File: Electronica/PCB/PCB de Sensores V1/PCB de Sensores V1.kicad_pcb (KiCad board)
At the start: 2 copper layers, 64.3 x 32.9 mm, 11 parts

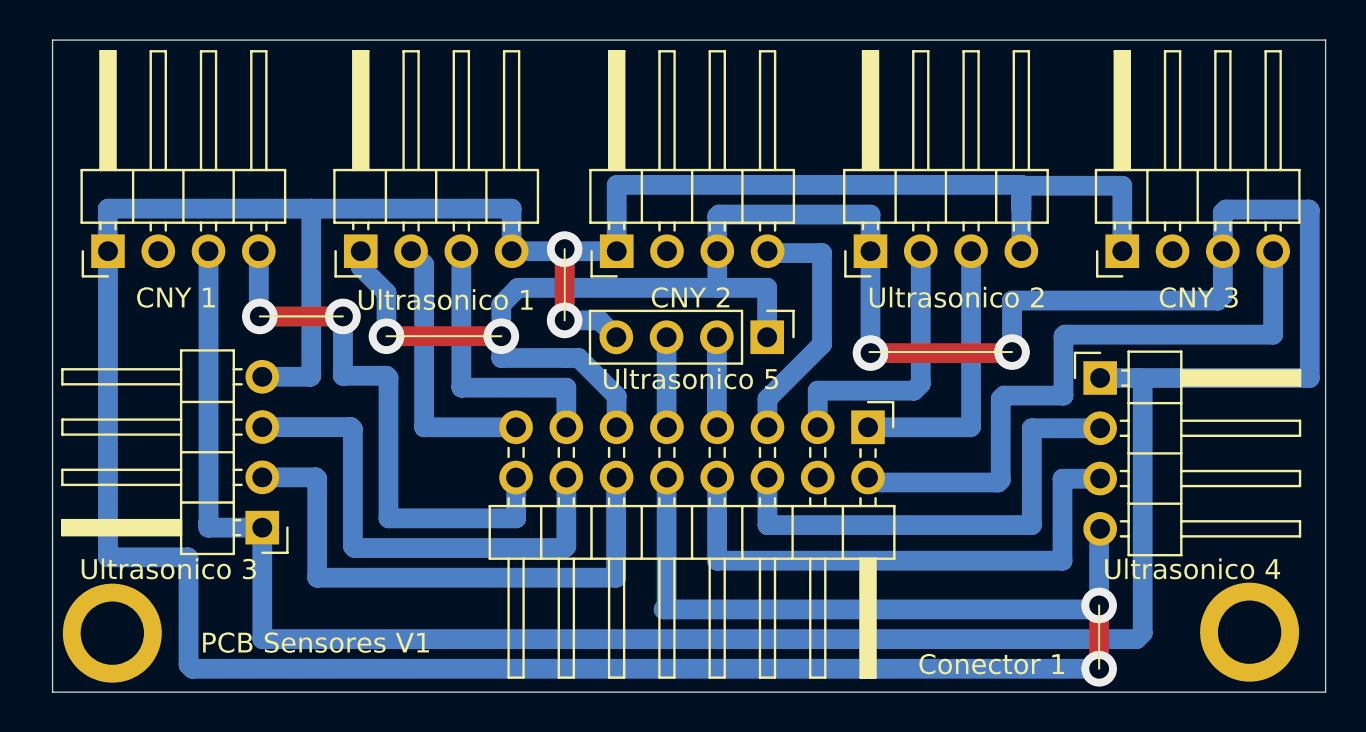
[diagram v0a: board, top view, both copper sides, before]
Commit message: ?
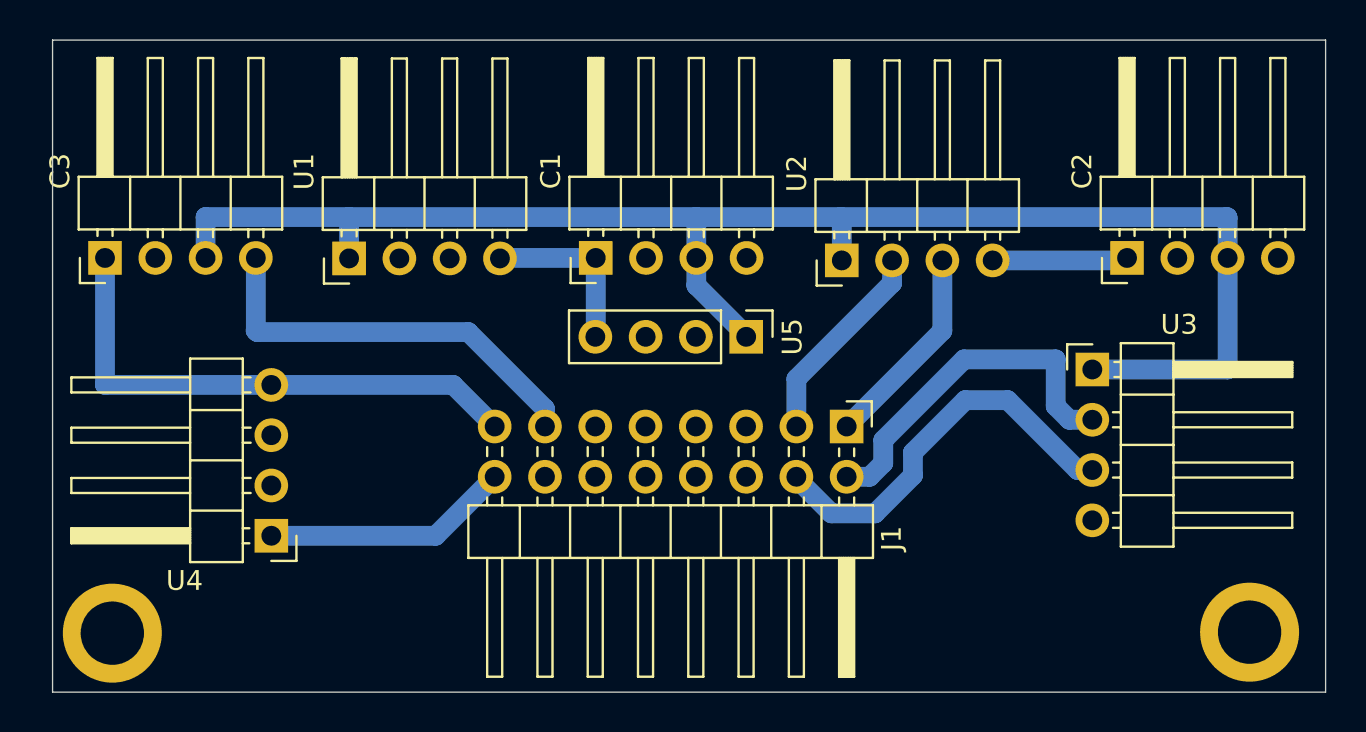
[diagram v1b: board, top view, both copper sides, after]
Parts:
- removed CNY 1: CNY1, Connector_PinHeader_2.54mm:PinHeader_1x04_P2.54mm_Horizontal
- removed CNY 2: CNY2, Connector_PinHeader_2.54mm:PinHeader_1x04_P2.54mm_Horizontal
- removed CNY 3: CNY3, Connector_PinHeader_2.54mm:PinHeader_1x04_P2.54mm_Horizontal
- removed Conector 1: Conn_02x08_Odd_Even, Connector_PinHeader_2.54mm:PinHeader_2x08_P2.54mm_Horizontal
- removed Ultrasonico 1: ULTRASONICO1, Connector_PinHeader_2.54mm:PinHeader_1x04_P2.54mm_Horizontal
- removed Ultrasonico 2: ULTRASONICO2, Connector_PinHeader_2.54mm:PinHeader_1x04_P2.54mm_Horizontal
- removed Ultrasonico 3: ULTRASONICO3, Connector_PinHeader_2.54mm:PinHeader_1x04_P2.54mm_Horizontal
- removed Ultrasonico 4: ULTRASONICO4, Connector_PinHeader_2.54mm:PinHeader_1x04_P2.54mm_Horizontal
- removed Ultrasonico 5: ULTRASONICO5, Connector_PinHeader_2.54mm:PinHeader_1x04_P2.54mm_Vertical
- added C1: CNY1, Connector_PinHeader_2.54mm:PinHeader_1x04_P2.54mm_Horizontal, F.Cu at (200.6, 53.2)
- added C2: CNY2, Connector_PinHeader_2.54mm:PinHeader_1x04_P2.54mm_Horizontal, F.Cu at (227.4, 53.2)
- added C3: CNY3, Connector_PinHeader_2.54mm:PinHeader_1x04_P2.54mm_Horizontal, F.Cu at (175.8, 53.2)
- added J1: Conexion Sensores, Connector_PinHeader_2.54mm:PinHeader_2x08_P2.54mm_Horizontal, F.Cu at (213.2, 61.8)
- added U1: ULTRASONICO1, Connector_PinHeader_2.54mm:PinHeader_1x04_P2.54mm_Horizontal, F.Cu at (188.1, 53.3)
- added U2: ULTRASONICO2, Connector_PinHeader_2.54mm:PinHeader_1x04_P2.54mm_Horizontal, F.Cu at (213.0, 53.4)
- added U3: ULTRASONICO3, Connector_PinHeader_2.54mm:PinHeader_1x04_P2.54mm_Horizontal, F.Cu at (225.7, 58.9)
- added U4: ULTRASONICO4, Connector_PinHeader_2.54mm:PinHeader_1x04_P2.54mm_Horizontal, F.Cu at (184.2, 67.3)
- added U5: ULTRASONICO5, Connector_PinHeader_2.54mm:PinHeader_1x04_P2.54mm_Vertical, F.Cu at (208.2, 57.2)
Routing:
- net +5V: track 191.5 -> 43.0 mm, vias 4 -> 0
- net GND: track 184.3 -> 92.1 mm, vias 4 -> 0
- net CNY3: track 31.8 -> 0.00 mm
- net CNY1: track 28.6 -> 0.00 mm, vias 2 -> 0
- net ECHO3: track 28.0 -> 0.00 mm
- net TRIG4: track 27.7 -> 0.00 mm
- net TRIG3: track 24.9 -> 0.00 mm
- net ECHO4: track 24.1 -> 0.00 mm
- net CNY 3: track 0.00 -> 20.8 mm
- net TRIG 3: track 0.00 -> 20.3 mm
- net ECHO 3: track 0.00 -> 18.2 mm
- net TRIG1: track 14.2 -> 0.00 mm
- net TRIG2: track 14.1 -> 0.00 mm
- net ECHO2: track 13.9 -> 0.00 mm
- net ECHO1: track 13.8 -> 0.00 mm
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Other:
- board text removed: "PCB Sensores V1"
